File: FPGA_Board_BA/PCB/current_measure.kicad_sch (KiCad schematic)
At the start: 4 parts, among them U3 AMC0300D, U4 AMC0300D, U5 AMC0300D, U6 AMC0300D

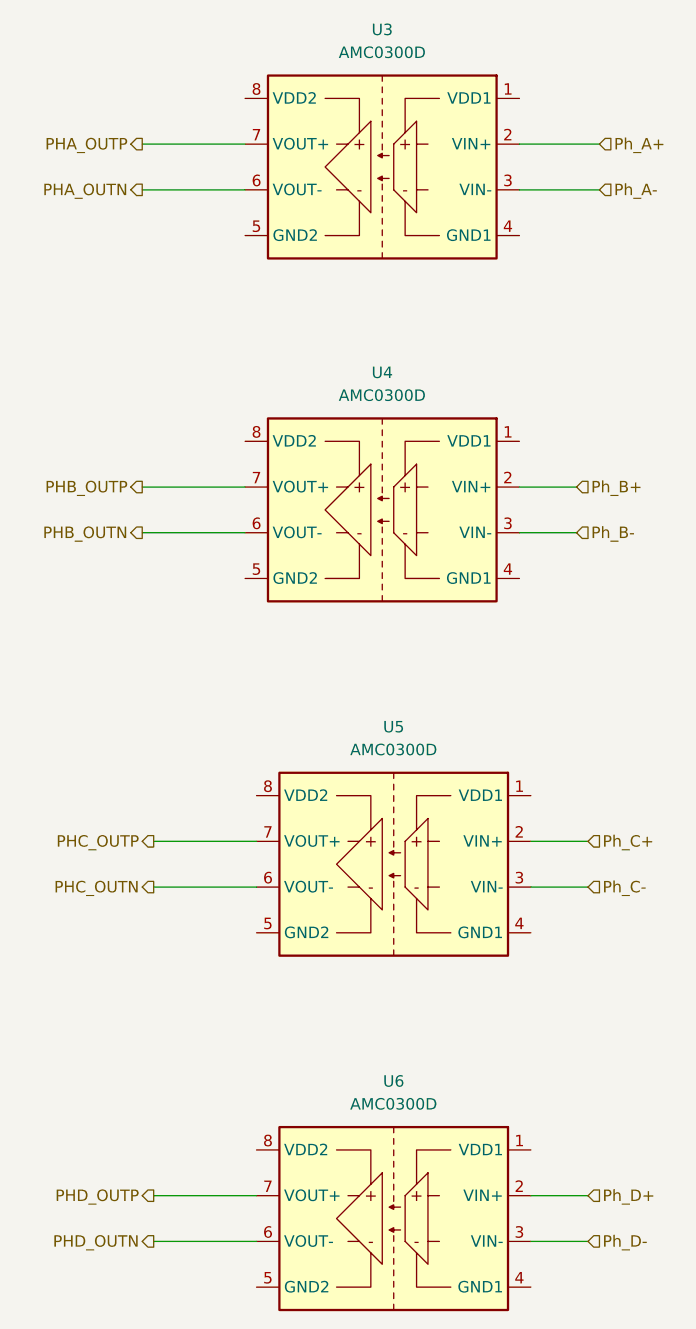
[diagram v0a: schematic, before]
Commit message: 22.11
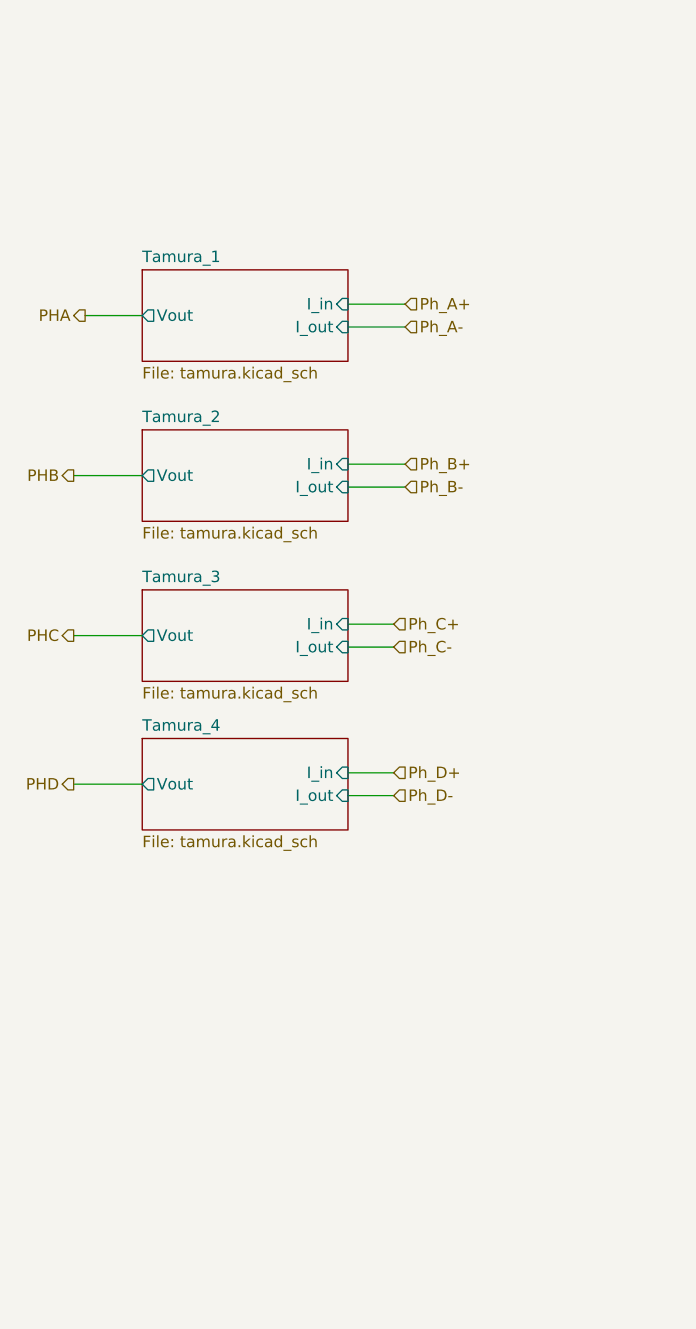
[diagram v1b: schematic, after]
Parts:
- removed U3, U4, U5, U6: AMC0300D, MYLIB_Misc:SOIC-8_7.5x5.85mm_P1.27mm, symbol MYLIB_Misc:AMC0300D
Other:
- added sheet Tamura_1 (tamura.kicad_sch)
- added sheet Tamura_2 (tamura.kicad_sch)
- added sheet Tamura_3 (tamura.kicad_sch)
- added sheet Tamura_4 (tamura.kicad_sch)
